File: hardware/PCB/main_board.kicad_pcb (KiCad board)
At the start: 2 copper layers, 72 x 100 mm, 49 parts, among them J1 TTL_UART, J10 POWER, J11 SDC_DEBUG, J12 UART_DEBUG, J2 DPS1_UART, J3 DPS2_UART, J4 PE_IO_0, J5 PE_IO_1, J6 PE_IO_2, J7 PE_IO_3/TWI0, J8 PA_IO, J9 USB_IO, Q1 2N3904(1AM), SW1 FEL, SW2 SW_Push, SW3 SW_Push, SW4 SW_Push, SW5 RESET, U1 TTL_USB_CONVERTER, U10 RTL8723BS, U11 100KΩ,(1003),±1%,0603,C25803, U12 10KΩ,(1002),±1%,0603,C25804, U13 M1,GPP,SMA,DO-214AC,C123825, U2 LICHEEPI_NANO, U3 47KΩ,(4702),±1%,0603,C25819, U4 47KΩ,(4702),±1%,0603,C25819, U5 47KΩ,(4702),±1%,0603,C25819, U6 47KΩ,(4702),±1%,0603,C25819, U7 47KΩ,(4702),±1%,0603,C25819, U8 33pF,(330),±5%,50V,C0G,0603,C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, U9 100KΩ,(1003),±1%,0603,C25803

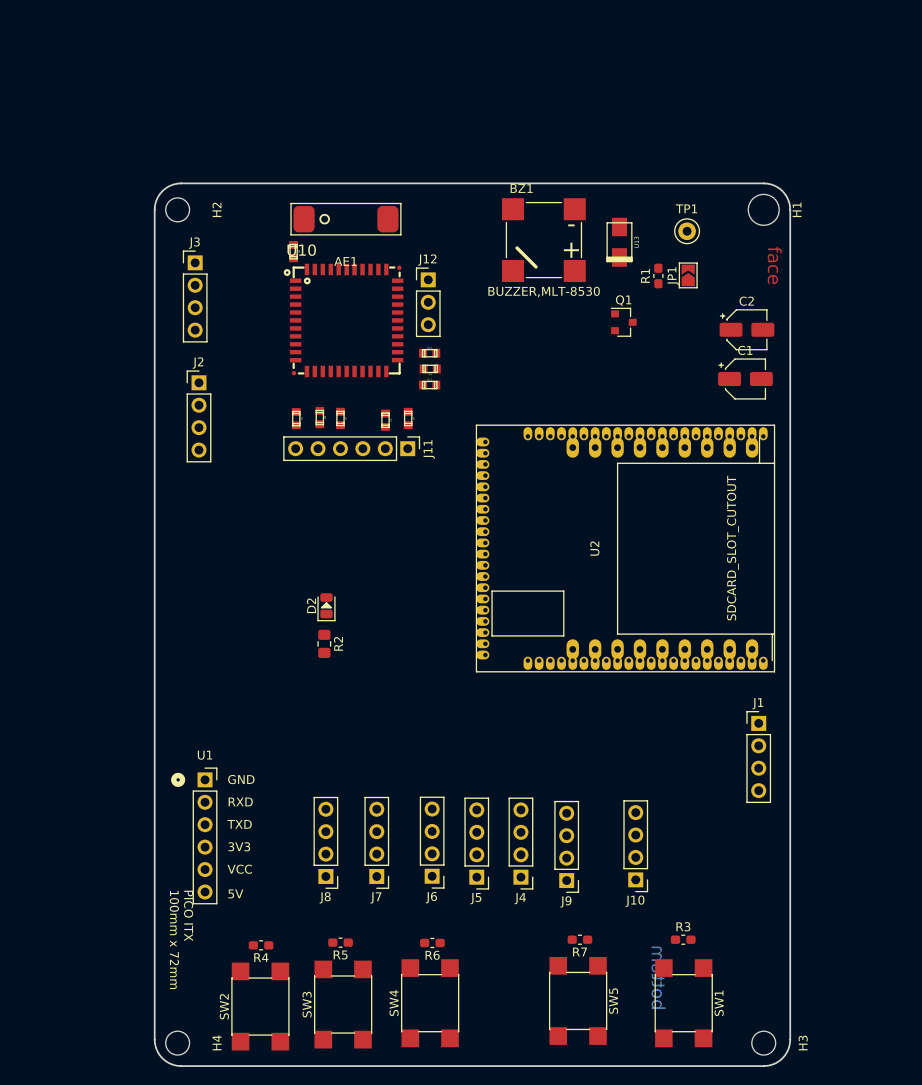
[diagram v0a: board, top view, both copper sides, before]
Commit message: update pcb mount,
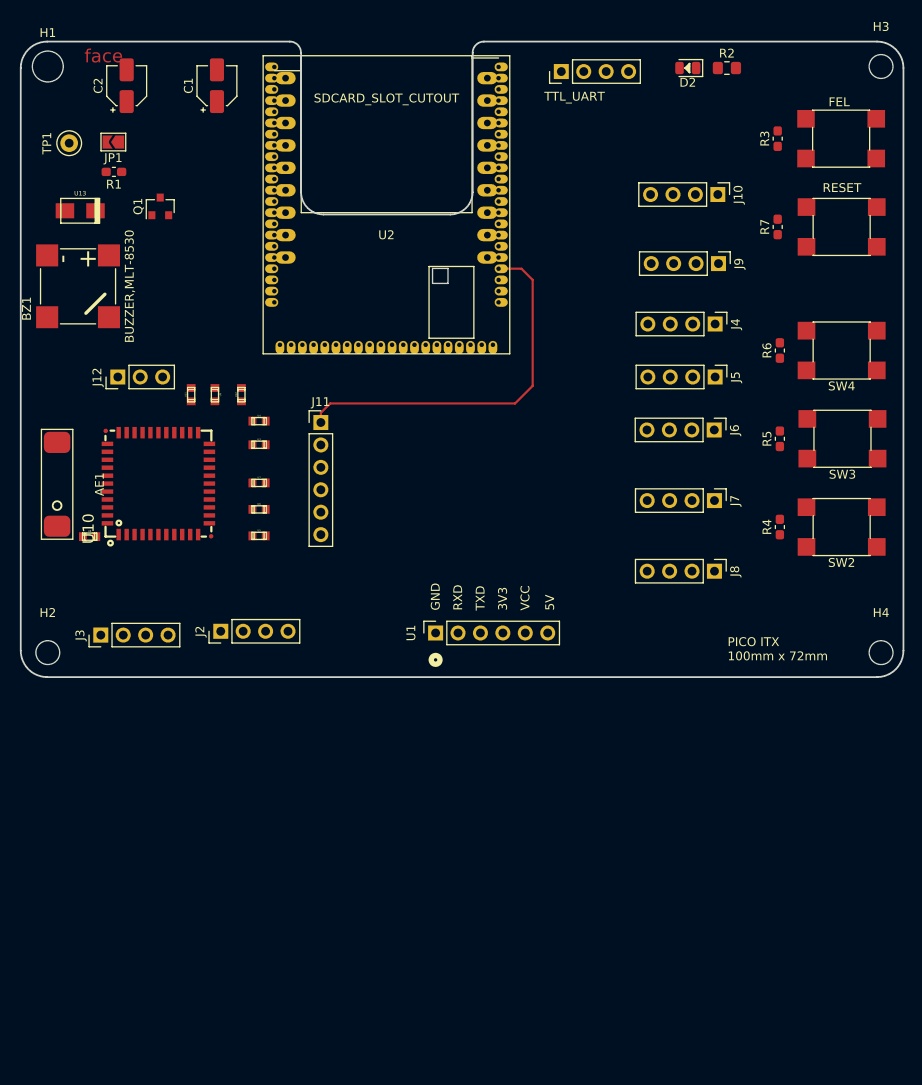
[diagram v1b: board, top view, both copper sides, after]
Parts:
- moved H3 111.4 mm to (97.5, 2.83), turned to 0 degrees
- moved SW1 99.6 mm to (92.9, 11.0), turned to 0 degrees
- moved SW5 92.6 mm to (93.0, 21.0), turned to 0 degrees
- moved R3 91.4 mm to (85.8, 11.0), turned to 90 degrees
- moved H4 91.1 mm to (97.5, 69.2), turned to 0 degrees
- moved SW4 87.4 mm to (93.0, 35.0), turned to 180 degrees
- moved SW3 85.5 mm to (93.1, 45.0), turned to 180 degrees
- moved SW2 85.4 mm to (93.0, 55.0), turned to 180 degrees
- moved R7 83.8 mm to (85.8, 21.0), turned to 90 degrees
- moved H1 82.7 mm to (3.07, 2.83), turned to 0 degrees
- moved R2 79.6 mm to (80.0, 3.00), turned to 0 degrees
- moved J10 78.2 mm to (79.0, 17.3), turned to 270 degrees
- moved R6 77.8 mm to (86.0, 35.0), turned to 90 degrees
- moved J1 77.2 mm to (61.2, 3.40), turned to 90 degrees
- moved R5 75.7 mm to (86.0, 45.0), turned to 90 degrees
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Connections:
- J5 pad 2: (no net) -> /PE5
- J5 pad 3: (no net) -> /PE6
- J6 pad 3: (no net) -> /PE10
- J7 pad 1: (no net) -> /I2C0-SCK
- J7 pad 2: (no net) -> /I2C0-SDA
- J8 pad 1: (no net) -> /PA0
- J8 pad 2: (no net) -> /PA1
- J9 pad 2: (no net) -> /USB_DM
- J9 pad 3: (no net) -> /USB_DP
- U2 pad 1: (no net) -> /USB_DM
- U2 pad 10: (no net) -> GND
- U2 pad 12: (no net) -> +3V3
- U2 pad 14: (no net) -> /PA0
- U2 pad 16: (no net) -> /PA1
- U2 pad 18: (no net) -> /PA2
- U2 pad 2: (no net) -> /PE2
- U2 pad 20: (no net) -> /PA3
- U2 pad 3: (no net) -> /USB_DP
- U2 pad 4: (no net) -> /PI_TTL_TXD
- U2 pad 45: (no net) -> /I2C0-SDA
- U2 pad 46: (no net) -> /SDC1_D1
- U2 pad 47: (no net) -> /I2C0-SCK
- U2 pad 48: (no net) -> /SDC1_D0
- U2 pad 49: (no net) -> /PE10
- U2 pad 50: (no net) -> /SDC1_CLK
- U2 pad 51: (no net) -> /PE9
- U2 pad 52: (no net) -> /SDC1_CMD
- U2 pad 53: (no net) -> /PE8
- U2 pad 54: (no net) -> /SDC1_D3
- U2 pad 55: (no net) -> /PE7
- U2 pad 56: (no net) -> /SDC1_D2
- U2 pad 57: (no net) -> /PE6
- U2 pad 58: (no net) -> /gpio/FEL
- U2 pad 59: (no net) -> /PE5
- U2 pad 6: (no net) -> /PI_TTL_RXD
- U2 pad 61: (no net) -> /PE4
- U2 pad 63: (no net) -> /PE3
- U2 pad 8: (no net) -> +5V
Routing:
- net /SDC1_D1: track 0.00 -> 42.8 mm
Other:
- board size 72 x 100 mm -> 100 x 72 mm
- board text removed: "bottom"
